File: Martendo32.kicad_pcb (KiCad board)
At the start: 2 copper layers, 75.2 x 98.5 mm, 107 parts, among them CN2 ZX-MX1.25-2PWT, J1 AudioJack4_SwitchTR1, J2 Conn_01x03, J4 USB-C, Q1 NPN, Q2 AO3401A, SW1 SK-3296S-01-L3, U3 TP4056, U4 NS4168, U5 TPS61040DBV, U6 AP2112K-3.3

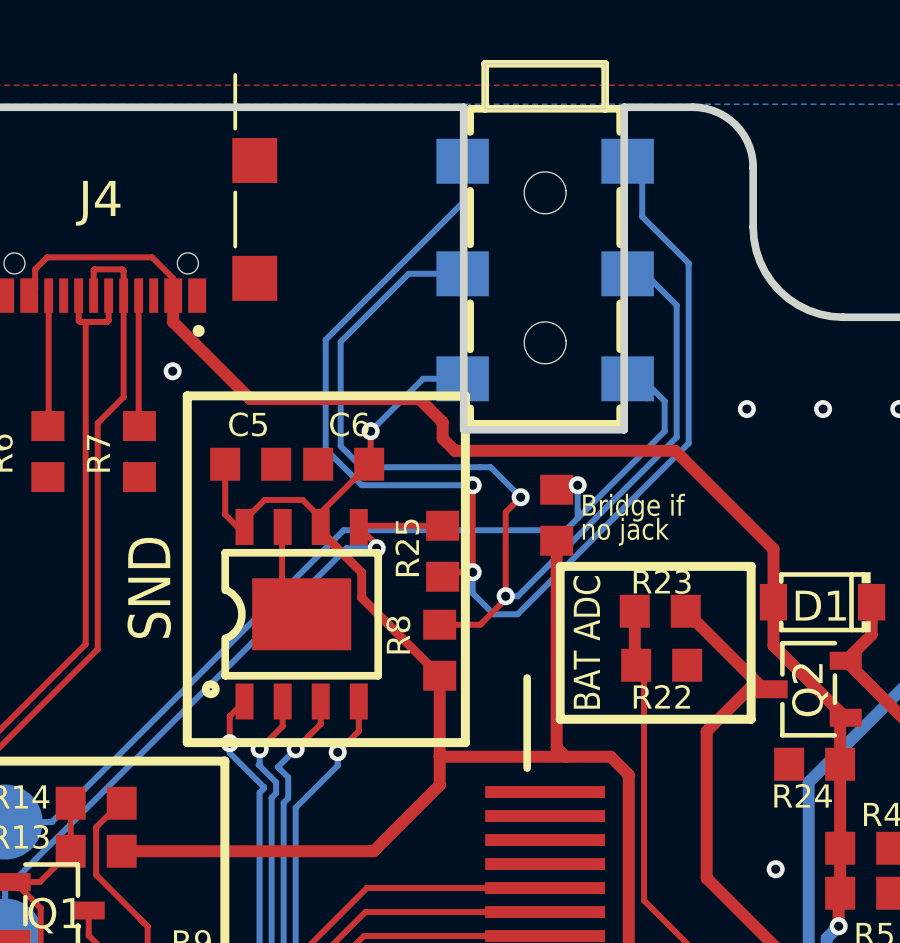
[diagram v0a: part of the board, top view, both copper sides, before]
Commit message: Add files via upload
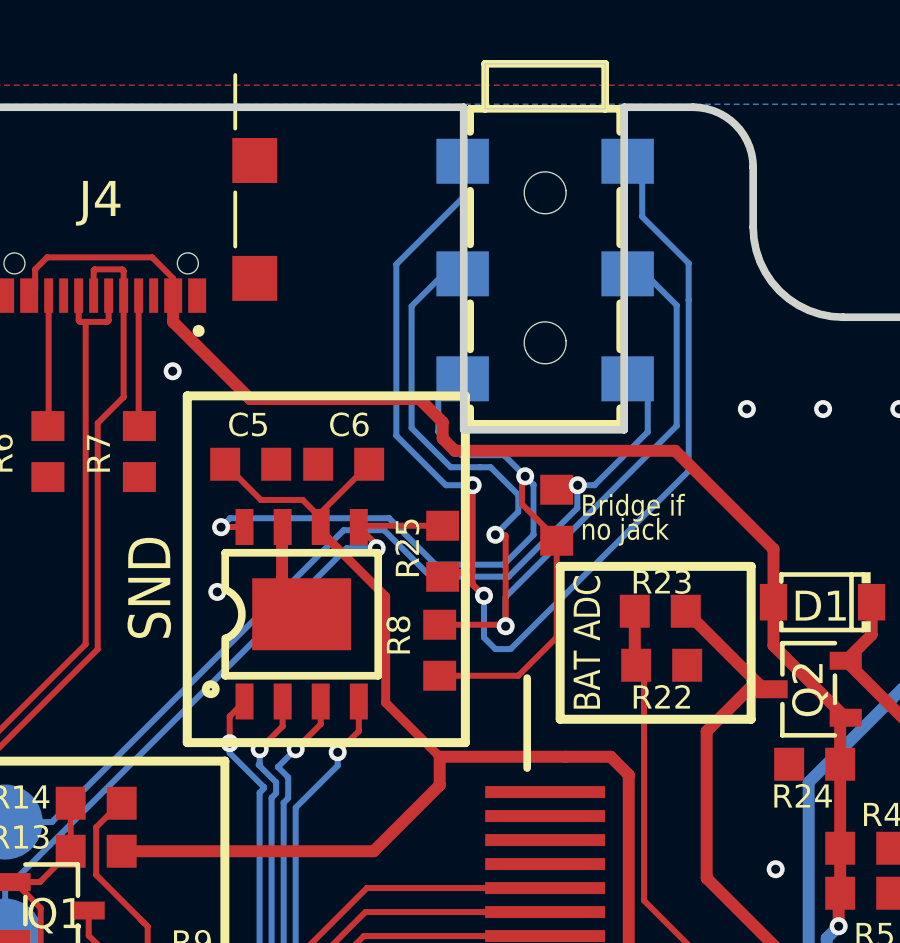
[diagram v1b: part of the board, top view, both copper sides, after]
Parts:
- R14, R25: value 10K -> 1K
- R21: value 10K -> 33k
- R4: value 2K -> 5K1
- R5: value 2K -> 1K
- R6, R7: value 10K -> 5K1
- R8: value 10K -> 240R
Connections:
- J1 pad TN: /+3V3 -> Net-(U4-VOP)
- R111 pad 1: /+3V3 -> Net-(U4-VOP)
- R8 pad 1: /+3V3 -> Net-(U4-VOP)
- U4 pad 8: /+3V3 -> Net-(U4-VOP)
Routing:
- net Net-(U4-VOP): track 0.00 -> 30.9 mm, vias 0 -> 2
- net /+3V3: track 280.1 -> 265.5 mm, vias 7 -> 6
- net /HPJ+1: track 35.2 -> 32.6 mm
- net /SPK1-: track 41.4 -> 40.7 mm
- net GND: vias 128 -> 129

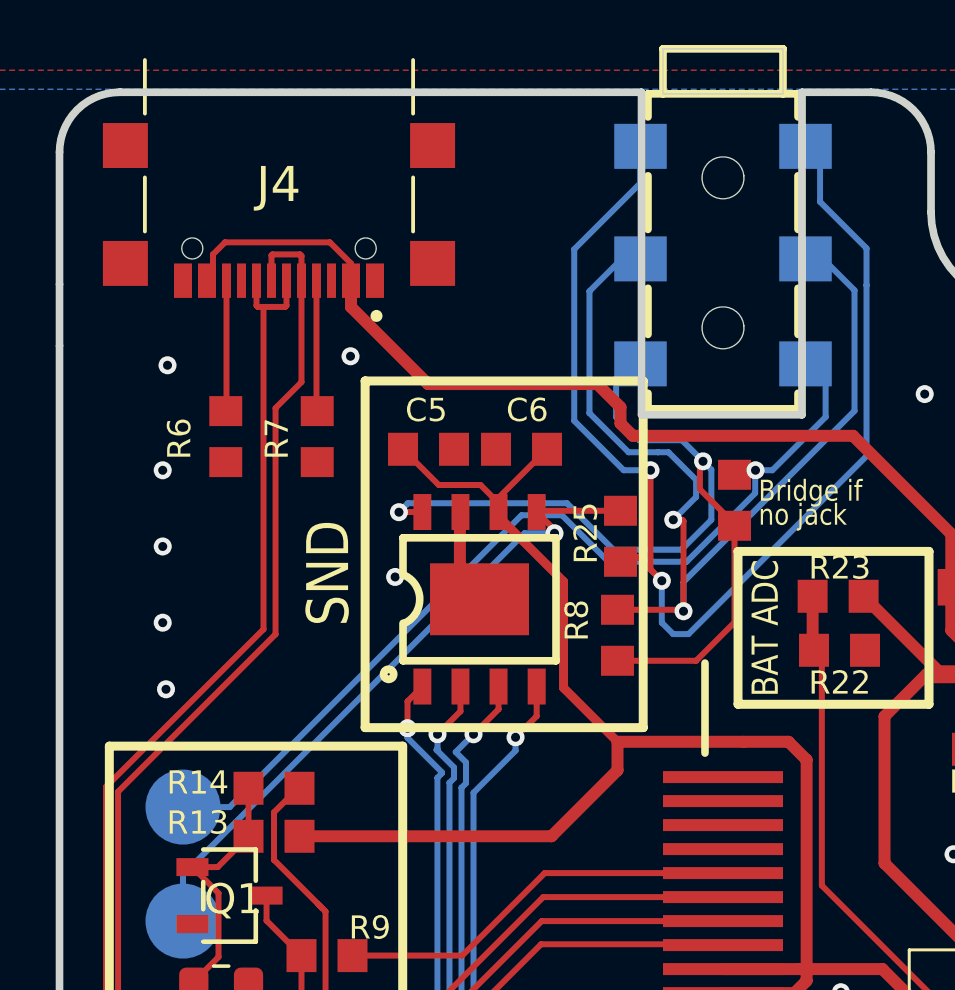
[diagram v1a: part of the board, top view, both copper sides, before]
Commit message: Add files via upload
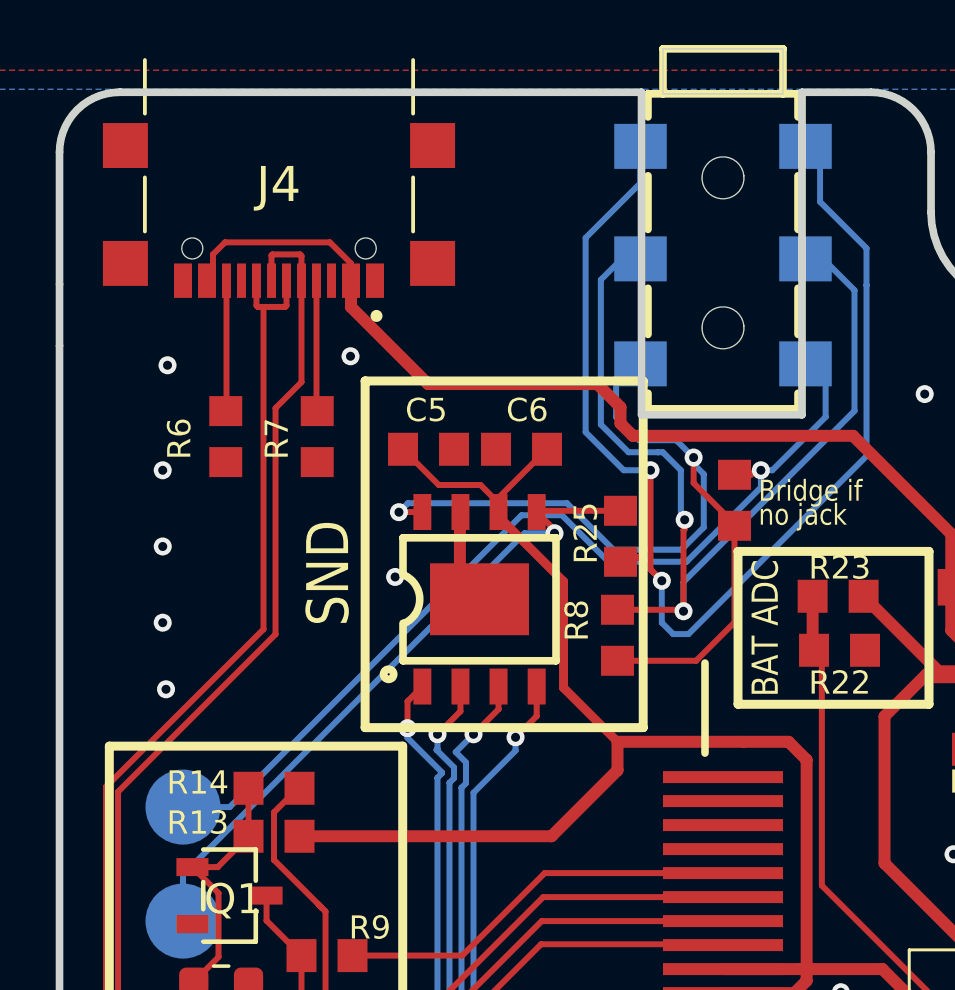
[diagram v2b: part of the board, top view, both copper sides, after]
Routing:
- net /HPJ+1: track 32.6 -> 31.4 mm
